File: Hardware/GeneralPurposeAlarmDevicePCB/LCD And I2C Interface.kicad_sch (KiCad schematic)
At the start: 32 parts, among them Q301 BSS138, U301 PCF8574AT_3_518, U302 LCD_20x4_Character-GPAD_SCH_L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

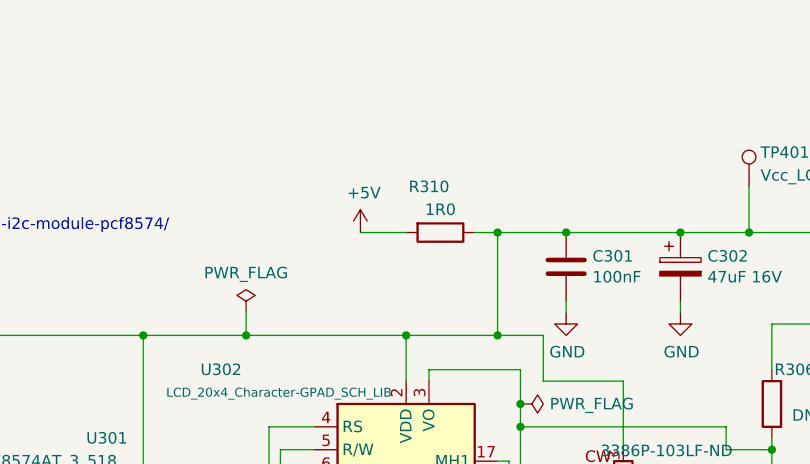
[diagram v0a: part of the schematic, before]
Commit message: Add Battery Control Circuitry
Added Battery Control Circuitry schematic as well as a MOSFET to turn on and off the LCD
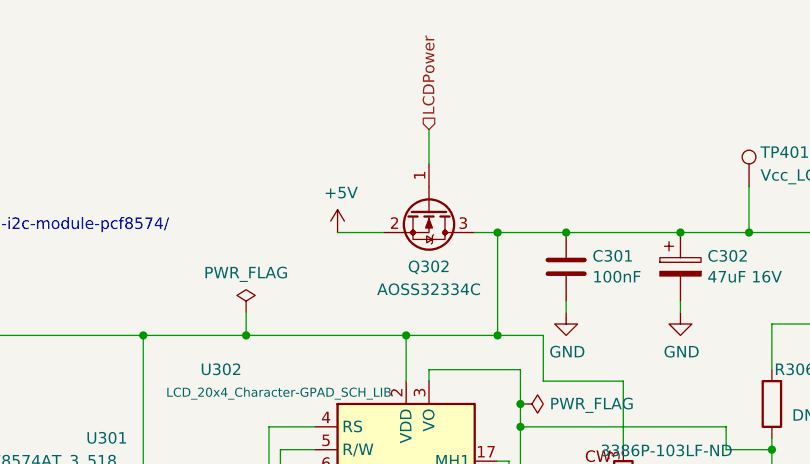
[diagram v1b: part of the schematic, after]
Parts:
- removed R310: 1R0, Resistor_SMD:R_0603_1608Metric_Pad0.98x0.95mm_HandSolder, symbol Device:R
- added Q302: AOSS32334C, Package_TO_SOT_SMD:SOT-23, symbol Transistor_FET:AO3400A
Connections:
- net +5V: now also Q302.2 (S)
- net Vcc_LCD: now also Q302.3 (D)
- new net LCDPower: Q302.1 (G)
